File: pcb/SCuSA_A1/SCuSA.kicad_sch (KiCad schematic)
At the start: 26 parts, among them J101 Header_01x02_Wurth_61300211121, J102 USB4135-GF-A, Q102 DMN2041LSD, SW101 SW_DPDT_x2, U1 LM27762, U101 MCP73812T-420I-OT, U102 AD8418, U103 BQ297xy

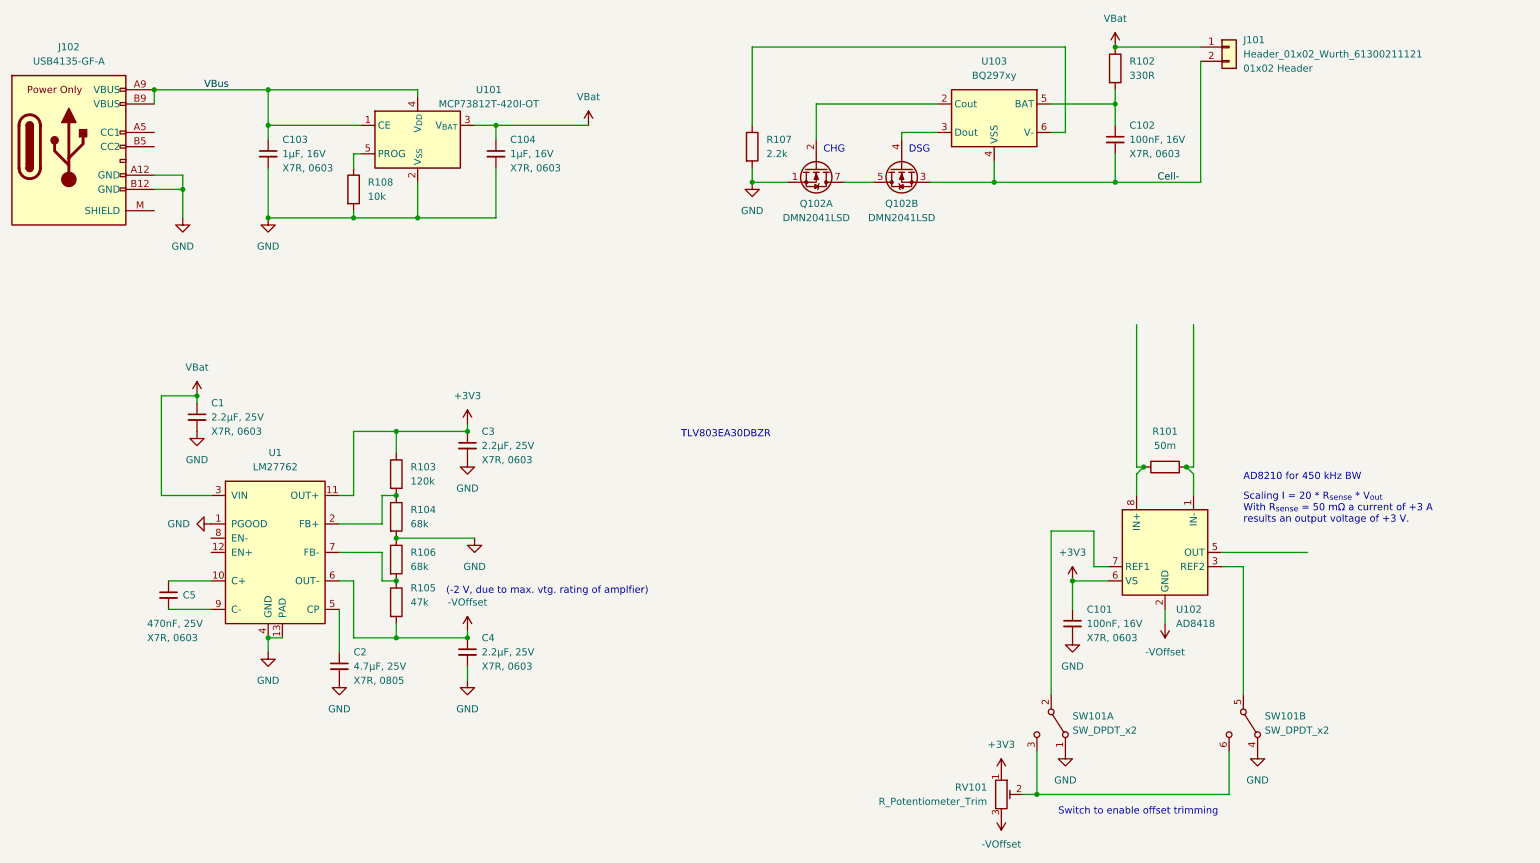
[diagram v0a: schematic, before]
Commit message: Work on battery charger
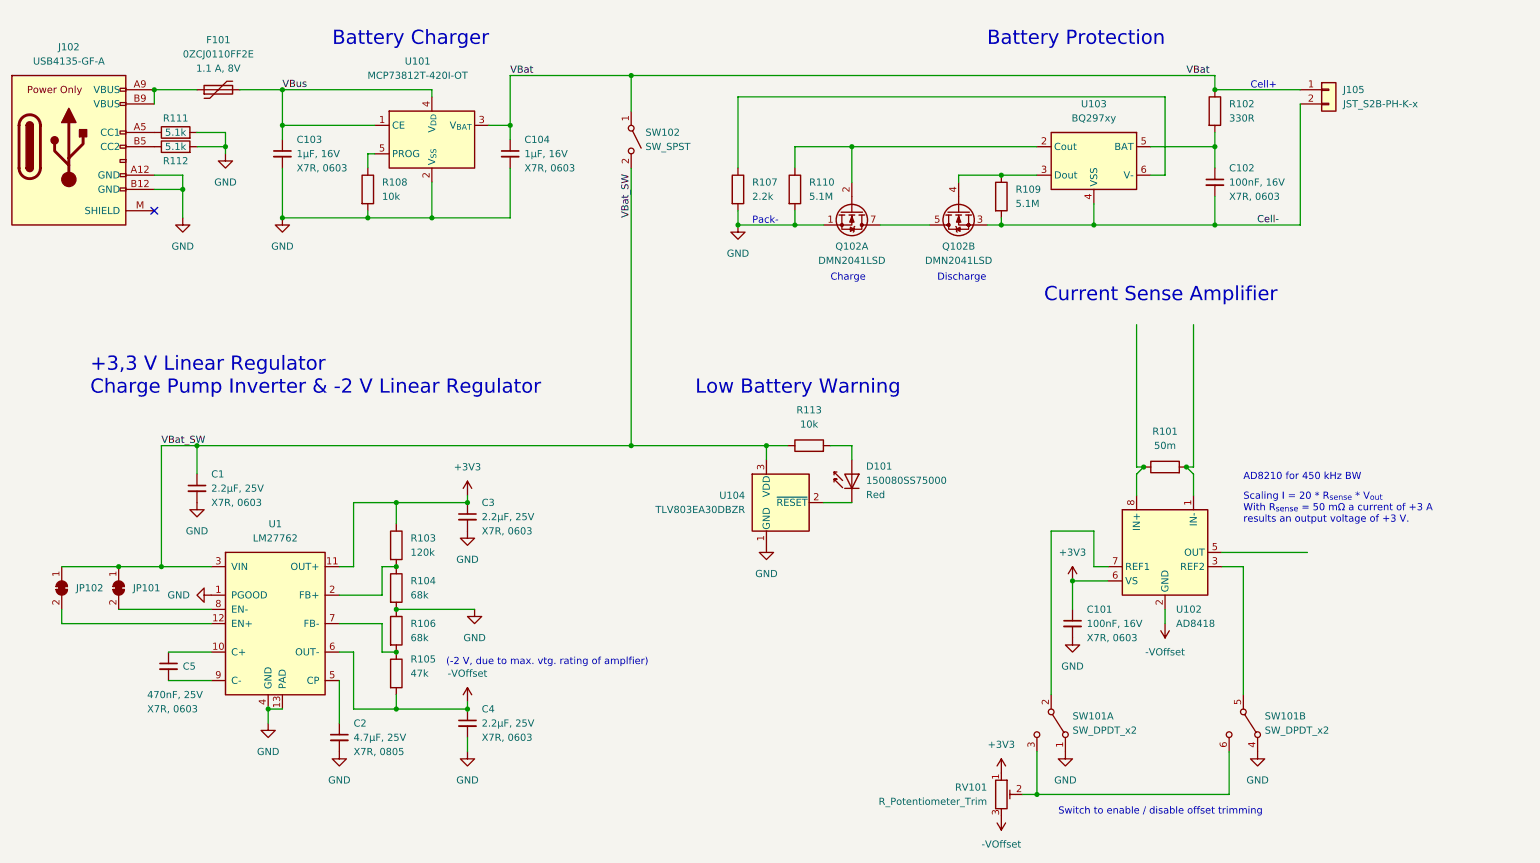
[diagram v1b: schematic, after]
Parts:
- removed J101: Header_01x02_Wurth_61300211121, Connector_PinHeader_2.54mm:PinHeader_1x02_P2.54mm_Vertical, symbol Connector_User:Header_01x02_Wurth_61300211121
- added D101: 150080SS75000, LED_SMD:LED_0805_2012Metric_Pad1.15x1.40mm_HandSolder, symbol LED_User:150080SS75000
- added F101: 0ZCJ0110FF2E, Fuse:Fuse_1206_3216Metric_Pad1.42x1.75mm_HandSolder, symbol Fuse_User:0ZCJ0110FF2E
- added J105: JST_S2B-PH-K-x, Connector_JST:JST_PH_S2B-PH-K_1x02_P2.00mm_Horizontal, symbol Connector_User:JST_S2B-PH-K-x
- added JP101, JP102: SolderJumper_2_Bridged, symbol Jumper:SolderJumper_2_Bridged
- added R109, R110: 5.1M,0603, Resistor_SMD:R_0603_1608Metric_Pad0.98x0.95mm_HandSolder, symbol Resistor_User:5.1M,0603
- added R111, R112: 5.1k,0603, Resistor_SMD:R_0603_1608Metric_Pad0.98x0.95mm_HandSolder, symbol Resistor_User:5.1k,0603
- added R113: 10k,0603, Resistor_SMD:R_0603_1608Metric_Pad0.98x0.95mm_HandSolder, symbol Resistor_User:10k,0603
- added SW102: SW_SPST, symbol Switch:SW_SPST
- added U104: TLV803EA30DBZR, Package_TO_SOT_SMD:SOT-23, symbol Power_Supervisor_User:TLV803EA30DBZR
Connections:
- net Cell-: now also J105.2 (Pin_2), R109.2
- net GND: now also R110.2, R111.2, R112.2, U104.1 (GND)
- net VBat: now also J105.1 (Pin_1), SW102.1 (A); no longer C1.1, U1.3 (VIN)
- net VBus: now also F101.2; no longer J102.A9 (VBUS), J102.B9 (VBUS)
- net at Q102.2 (G1), U103.2 (Cout): now also R110.1
- net at Q102.4 (G2), U103.3 (Dout): now also R109.1
- net at U1.12 (EN+): now also JP102.2 (B)
- net at U1.8 (EN-): now also JP101.2 (B)
- net at J102.A5 (CC1): now also R111.1
- net at J102.B5 (CC2): now also R112.1
- new net: D101.2 (A), R113.2
- new net: D101.1 (K), U104.2 (~{RESET})
- new net: F101.1, J102.A9 (VBUS), J102.B9 (VBUS)
- new net VBat_SW: C1.1, JP101.1 (A), JP102.1 (A), R113.1, SW102.2 (B), U1.3 (VIN), U104.3 (VDD)
- no-connect marks 0 -> 1
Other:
- note added: "+3,3 V Linear Regulator Charge Pump Inverter & -2 V Linear Regulator"
- note added: "Battery Charger"
- note added: "Battery Protection"
- note added: "Cell+"
- note added: "Charge"
- note added: "Current Sense Amplifier"
- note added: "Discharge"
- note added: "Low Battery Warning"
- note added: "Pack-"
- note added: "Switch to enable / disable offset trimming"
- note removed: "CHG"
- note removed: "DSG"
- note removed: "Switch to enable offset trimming"
- note removed: "TLV803EA30DBZR"
- moved on the sheet: C1, C102, C103, C104, C2, C3, C4, C5, Q102A, Q102B, R102, R103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
